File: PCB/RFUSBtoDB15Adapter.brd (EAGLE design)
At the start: 52.1 x 68.6 mm, 24 parts, among them IC1 S-816A40AMC-BAPT2U, J1 0, J2 AVR_SPI_PROG_3X2NS, Q2 2SA1213-Y(TE12L,F)

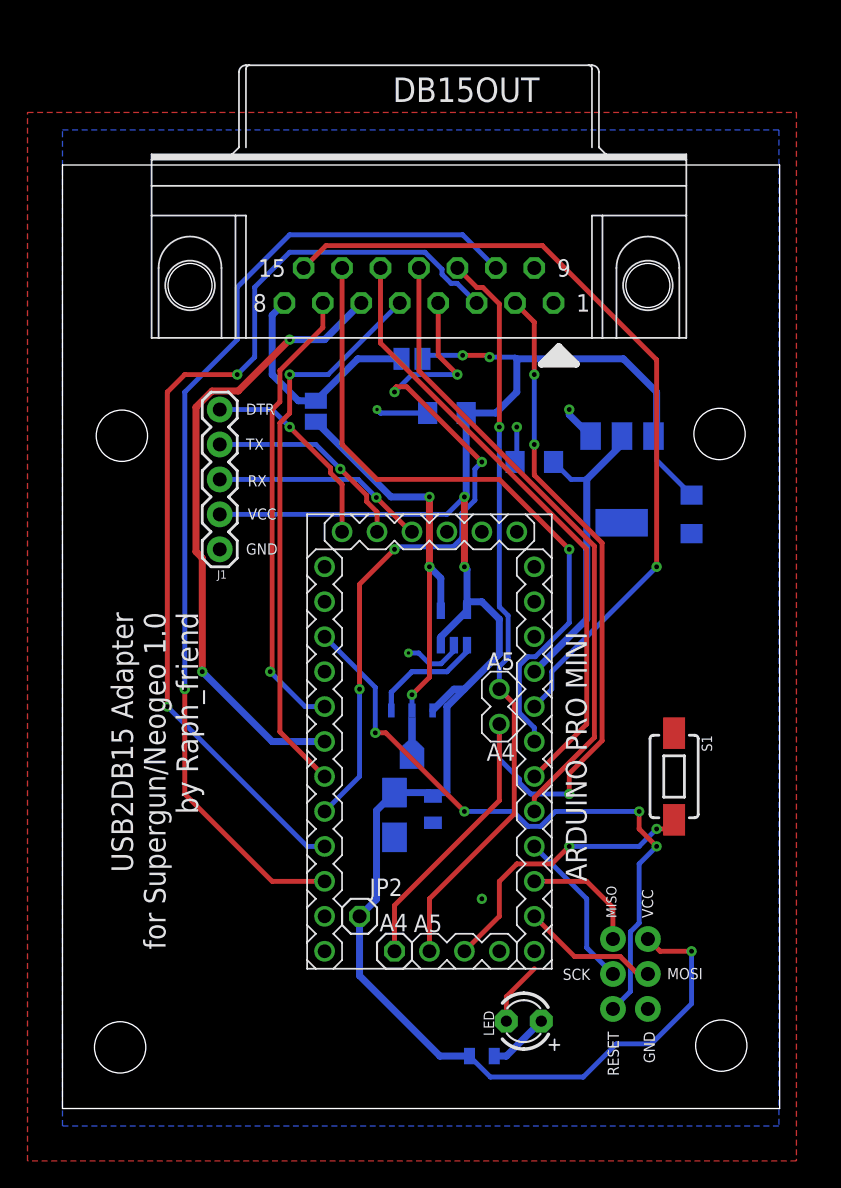
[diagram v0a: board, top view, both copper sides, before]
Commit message: PCB Update
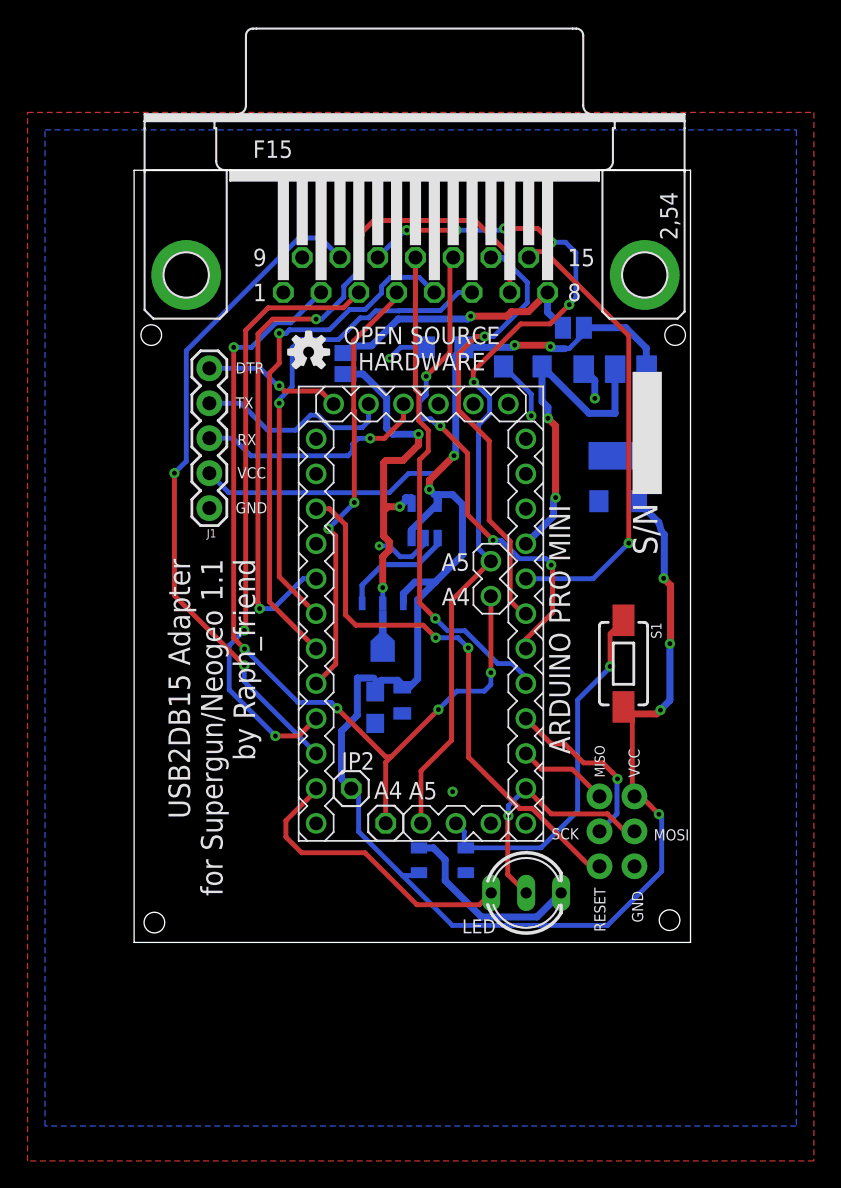
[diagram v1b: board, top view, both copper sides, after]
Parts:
- removed DB15OUT: 0, dbconnector:D-15M/90
- removed PEM1, PEM2, PEM3, PEM4: KF2-M2, penn-engineering:KF2-M2
- removed R1: 80R, SparkFun-Resistors:0805
- added R2: 10K, SparkFun-Resistors:0805
- added R3: 500R, SparkFun-Resistors:0805
- added U$2: (no value), RF_logo:RF_LOGO
- added X1: (no value), con-subd:F15HP
- C5: value 4.7UF -> 4.7uf; device resistor:B/3528-21W -> tantalum cap:CAPMP3.4X1.6_1.8N_KEM
- LED: value (none) -> led; device adafruit:LED3MM -> led:DUOLED-C-5MM
- moved LOGO1 18.6 mm to (15.4, 66.4), flipped to the top, turned to 0 degrees
- moved SJ1 12.0 mm to (34.6, 68.2)
- moved J2 10.4 mm to (37.8, 31.6)
- moved A4 9.33 mm to (20.9, 32.2)
- moved LED 9.32 mm to (31.2, 27.1), turned to 0 degrees
- moved ARDUINO-MINIPRO 9.31 mm to (23.5, 47.4)
- moved JP2 9.30 mm to (18.4, 34.7)
- moved S1 8.99 mm to (38.2, 43.8)
- moved C1 8.25 mm to (22.2, 41.1)
- moved IC1 8.07 mm to (23.8, 54.1)
- moved Q2 8.07 mm to (20.7, 46.4)
- moved C5 7.93 mm to (20.2, 40.6), turned to 270 degrees
- moved C4 7.00 mm to (30.9, 65.4)
- moved C3 5.42 mm to (37.8, 55.6), turned to 180 degrees
- moved 3.3V 4.89 mm to (37.6, 62.0)
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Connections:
- removed net 5VLED: LED.A, R1.1
- new net LEDREG: LED.AR, R3.2
- new net N$8: X1.9
- net 5VREG: now also C5.1, R3.1, S1.2; no longer C5.+, R1.2
- net 5VSG: now also X1.8; no longer DB15OUT.8
- net BUT1: now also X1.13; no longer DB15OUT.13
- net BUT2: now also X1.5; no longer DB15OUT.5
- net BUT3: now also X1.12; no longer DB15OUT.12
- net BUT4: now also X1.4; no longer DB15OUT.4
- net BUT5: now also X1.10; no longer DB15OUT.10
- net BUT6: now also X1.2; no longer DB15OUT.2
- net CREDIT: now also X1.3; no longer DB15OUT.3
- net DOWN: now also X1.7; no longer DB15OUT.7
- net GND: now also C5.2, R2.1, X1.1; no longer C5.-, DB15OUT.1, S1.1
- net LED: now also LED.AX; no longer LED.K
- net LEFT: now also X1.14; no longer DB15OUT.14
- net MOSI: now also LED.C
- net RESET_MEM: now also R2.2, S1.1; no longer S1.2
- net RIGHT: now also X1.6; no longer DB15OUT.6
- net START: now also X1.11; no longer DB15OUT.11
- net UP: now also X1.15; no longer DB15OUT.15
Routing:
- net CREDIT: track 69.9 -> 44.2 mm
- net UP: track 58.7 -> 33.6 mm
- net BUT5: track 72.6 -> 49.1 mm, vias 1 -> 2
- net BUT4: track 52.3 -> 31.3 mm, vias 5 -> 2
- net DOWN: track 33.5 -> 52.5 mm, vias 1 -> 3
- net LED: track 4.65 -> 21.8 mm
- net LEFT: track 48.7 -> 32.4 mm
- net LEDREG: track 0.00 -> 14.0 mm
- net START: track 54.7 -> 65.3 mm, vias 1 -> 6
- net BUT3: track 46.6 -> 36.2 mm, vias 0 -> 1
- net RIGHT: track 45.6 -> 35.6 mm, vias 2 -> 1
- net BUT1: track 44.7 -> 36.1 mm, vias 0 -> 4
- net MOSI: track 9.99 -> 17.9 mm, vias 0 -> 1
- net RESET: track 47.1 -> 39.8 mm, vias 4 -> 2
- net RESET_MEM: track 20.7 -> 26.6 mm, vias 2 -> 1
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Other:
- board size 52.1 x 68.6 mm -> 40.4 x 56.1 mm
- board text added: "OPEN SOURCE HARDWARE"
- board text added: "S/N"
- board text added: "USB2DB15 Adapter for Supergun/Neogeo 1.1 by Raph_friend"
- board text removed: "4.7uf"
- board text removed: "USB2DB15 Adapter for Supergun/Neogeo 1.0 by Raph_friend"
